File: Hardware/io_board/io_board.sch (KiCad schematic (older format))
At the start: 30 parts, among them J1 Conn_01x40, J2 Conn_02x05_Odd_Even, J3 Mini-DIN-6, J4 Conn_02x10_Odd_Even, U1 74LS138, U2 W65C22NxP, U3 74LS14

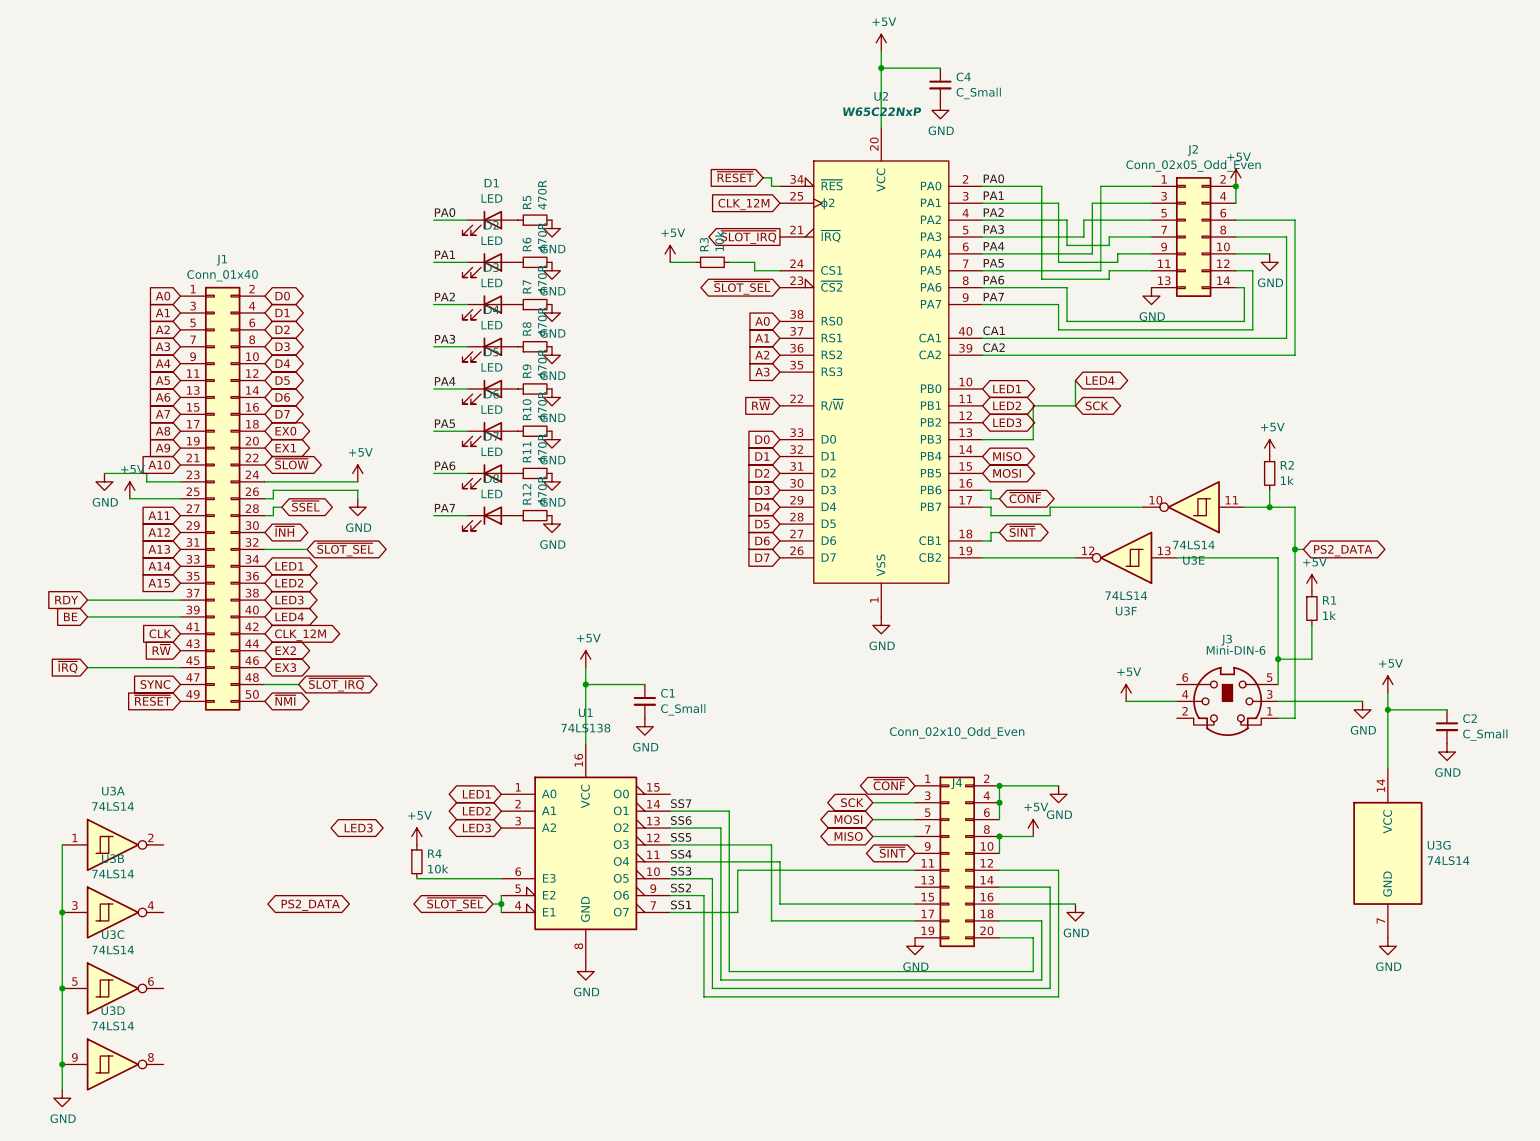
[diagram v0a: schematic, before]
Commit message: small fixes on the hardware
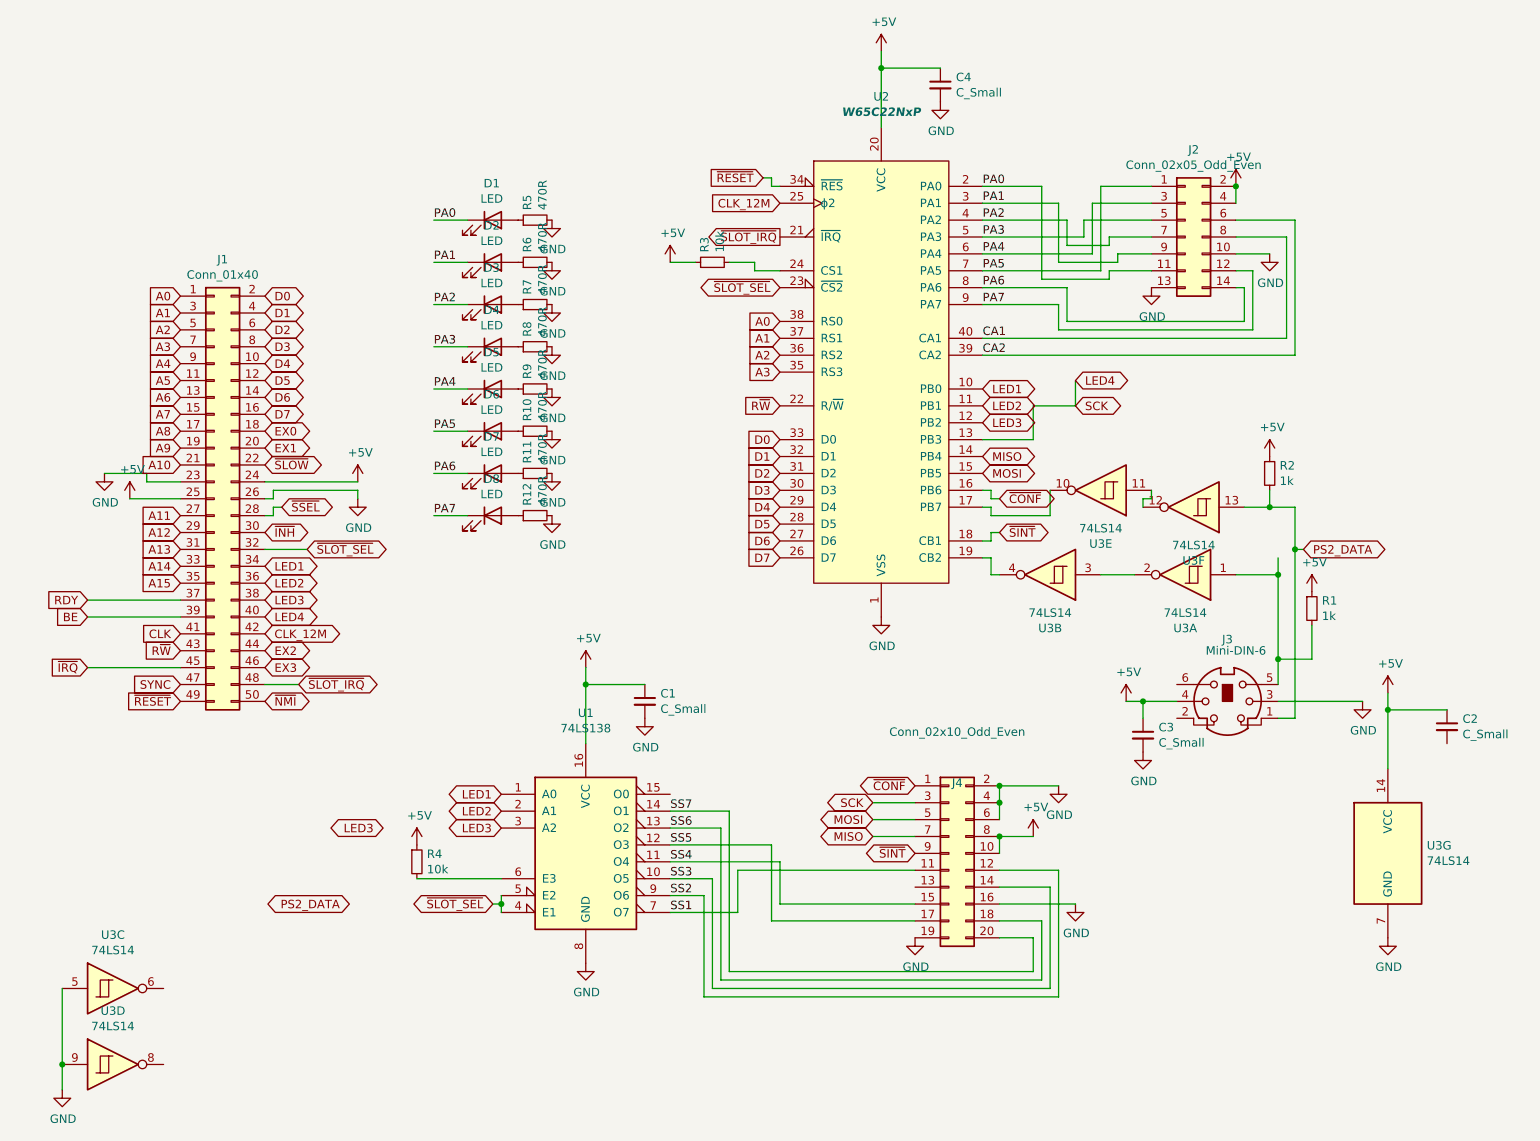
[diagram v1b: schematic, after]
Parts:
- added C3: C_Small, Capacitor_SMD:C_1206_3216Metric_Pad1.42x1.75mm_HandSolder, symbol Device:C_Small
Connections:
- net +5V: now also C3.1
- net GND: now also C3.2; no longer C2.2, U3.1, U3.3
- net PS2_DATA: now also U3.13; no longer U3.11
- net at U2.19 (CB2): now also U3.4; no longer U3.12
- net at J3.5, R1.2: now also U3.1; no longer U3.13
- net at U3.2: now also U3.3
- new net: U3.11, U3.12
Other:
- moved on the sheet: U3A, U3B, U3E, U3F
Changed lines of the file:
@@
 $EndComp
 Wire Wire Line
-	8200 4650 7900 4650
+	8200 4650 8000 4650
 Wire Wire Line
 	8800 4750 8900 4750
@@
 	7100 3400 7050 3400
 Wire Wire Line
-	7450 3500 7450 3550
-Wire Wire Line
 	7450 3550 7100 3550
 Wire Wire Line
@@
 L 74xx:74LS14 U3
 U 1 1 601A49CD
-P 1900 5500
-F 0 "U3" H 1900 5817 50  0000 C CNN
-F 1 "74LS14" H 1900 5726 50  0000 C CNN
-F 2 "Package_DIP:DIP-14_W7.62mm_Socket" H 1900 5500 50  0001 C CNN
-F 3 "http://www.ti.com/lit/gpn/sn74LS14" H 1900 5500 50  0001 C CNN
-	1    1900 5500
-	1    0    0    -1
+P 8250 3900
+F 0 "U3" H 8250 4217 50  0000 C CNN
+F 1 "74LS14" H 8250 4126 50  0000 C CNN
+F 2 "Package_DIP:DIP-14_W7.62mm_Socket" H 8250 3900 50  0001 C CNN
+F 3 "http://www.ti.com/lit/gpn/sn74LS14" H 8250 3900 50  0001 C CNN
+	1    8250 3900
+	-1   0    0    1
 $EndComp
 $Comp
 L 74xx:74LS14 U3
 U 2 1 601A559B
-P 1900 5900
-F 0 "U3" H 1900 6217 50  0000 C CNN
-F 1 "74LS14" H 1900 6126 50  0000 C CNN
-F 2 "Package_DIP:DIP-14_W7.62mm_Socket" H 1900 5900 50  0001 C CNN
-F 3 "http://www.ti.com/lit/gpn/sn74LS14" H 1900 5900 50  0001 C CNN
-	2    1900 5900
-	1    0    0    -1
+P 7450 3900
+F 0 "U3" H 7450 4217 50  0000 C CNN
+F 1 "74LS14" H 7450 4126 50  0000 C CNN
+F 2 "Package_DIP:DIP-14_W7.62mm_Socket" H 7450 3900 50  0001 C CNN
+F 3 "http://www.ti.com/lit/gpn/sn74LS14" H 7450 3900 50  0001 C CNN
+	2    7450 3900
+	-1   0    0    1
 $EndComp
 $Comp
@@
 L 74xx:74LS14 U3
 U 5 1 601A824E
+P 7750 3400
+F 0 "U3" H 7750 3717 50  0000 C CNN
+F 1 "74LS14" H 7750 3626 50  0000 C CNN
+F 2 "Package_DIP:DIP-14_W7.62mm_Socket" H 7750 3400 50  0001 C CNN
+F 3 "http://www.ti.com/lit/gpn/sn74LS14" H 7750 3400 50  0001 C CNN
+	5    7750 3400
+	-1   0    0    1
+$EndComp
+$Comp
+L 74xx:74LS14 U3
+U 6 1 601A8ACA
 P 8300 3500
 F 0 "U3" H 8300 3817 50  0000 C CNN
@@
 F 2 "Package_DIP:DIP-14_W7.62mm_Socket" H 8300 3500 50  0001 C CNN
 F 3 "http://www.ti.com/lit/gpn/sn74LS14" H 8300 3500 50  0001 C CNN
-	5    8300 3500
-	-1   0    0    1
-$EndComp
-$Comp
-L 74xx:74LS14 U3
-U 6 1 601A8ACA
-P 7900 3800
-F 0 "U3" H 7900 4117 50  0000 C CNN
-F 1 "74LS14" H 7900 4026 50  0000 C CNN
-F 2 "Package_DIP:DIP-14_W7.62mm_Socket" H 7900 3800 50  0001 C CNN
-F 3 "http://www.ti.com/lit/gpn/sn74LS14" H 7900 3800 50  0001 C CNN
-	6    7900 3800
+	6    8300 3500
 	-1   0    0    1
 $EndComp
@@
 	8900 3500 8750 3500
 Wire Wire Line
-	7450 3500 8000 3500
-Wire Wire Line
 	8750 3400 8750 3500
 Connection ~ 8750 3500
@@
 Connection ~ 8800 4400
 Wire Wire Line
-	8800 4400 8800 3800
-Wire Wire Line
-	8800 3800 8200 3800
-Wire Wire Line
-	7050 3800 7600 3800
+	8800 4400 8800 3900
 $Comp
 L power:+5V #PWR0132
@@
 L power:GND #PWR0133
 U 1 1 6023E74F
-P 9800 4900
-F 0 "#PWR0133" H 9800 4650 50  0001 C CNN
-F 1 "GND" H 9805 4727 50  0000 C CNN
-F 2 "" H 9800 4900 50  0001 C CNN
-F 3 "" H 9800 4900 50  0001 C CNN
-	1    9800 4900
+P 8000 4950
+F 0 "#PWR0133" H 8000 4700 50  0001 C CNN
+F 1 "GND" H 8005 4777 50  0000 C CNN
+F 2 "" H 8000 4950 50  0001 C CNN
+F 3 "" H 8000 4950 50  0001 C CNN
+	1    8000 4950
 	1    0    0    -1
 $EndComp
@@
 $EndComp
 Wire Wire Line
-	1600 5500 1600 5900
-Connection ~ 1600 5900
-Wire Wire Line
-	1600 5900 1600 6350
-Connection ~ 1600 6350
-Wire Wire Line
 	1600 6350 1600 6800
 Connection ~ 1600 6800
@@
 	4200 5900 4200 5850
 Connection ~ 4200 5850
+$Comp
+L Device:C_Small C3
+U 1 1 604850AB
+P 8000 4850
+F 0 "C3" H 8092 4896 50  0000 L CNN
+F 1 "C_Small" H 8092 4805 50  0000 L CNN
+F 2 "Capacitor_SMD:C_1206_3216Metric_Pad1.42x1.75mm_HandSolder" H 8000 4850 50  0001 C CNN
+F 3 "~" H 8000 4850 50  0001 C CNN
+	1    8000 4850
+	1    0    0    -1
+$EndComp
+Wire Wire Line
+	8000 4750 8000 4650
+Connection ~ 8000 4650
+Wire Wire Line
+	8000 4650 7900 4650
+Wire Wire Line
+	8050 3400 8050 3450
+Wire Wire Line
+	8050 3450 8000 3450
+Wire Wire Line
+	8000 3450 8000 3500
+Wire Wire Line
+	7450 3400 7450 3550
+Wire Wire Line
+	8550 3900 8800 3900
+Connection ~ 8800 3900
+Wire Wire Line
+	8800 3900 8800 3800
+Wire Wire Line
+	7950 3900 7750 3900
+Wire Wire Line
+	7150 3900 7100 3900
+Wire Wire Line
+	7100 3900 7100 3800
+Wire Wire Line
+	7100 3800 7050 3800
 $EndSCHEMATC
